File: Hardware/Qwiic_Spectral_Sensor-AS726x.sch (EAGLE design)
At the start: 29 parts, among them J1 Qwiic Right Angle, J2 Serial Interface, J4 Qwiic Right Angle, J5 Flash Programming, U1 IR, U3 4MB Flash

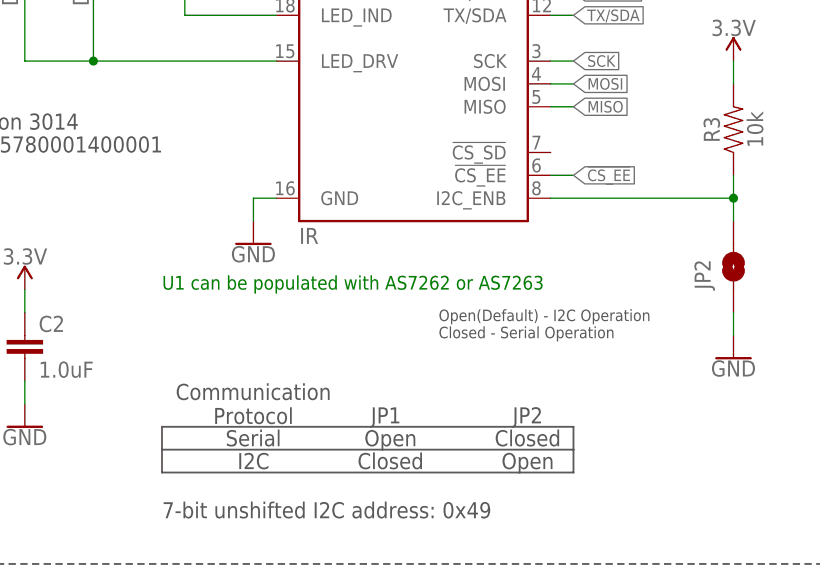
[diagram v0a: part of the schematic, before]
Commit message: Fixed minor borad layout issues
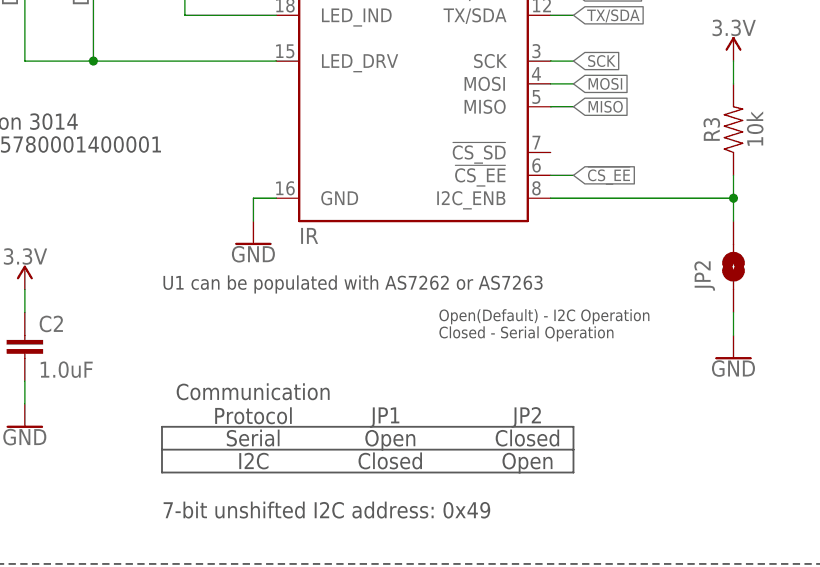
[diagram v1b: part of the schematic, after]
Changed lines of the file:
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@@
 Reset</text>
 <text x="148.59" y="7.112" size="2.54" layer="95">Revised by: Andy England</text>
-<text x="48.26" y="106.68" size="1.524" layer="91">U1 can be populated with AS7262 or AS7263</text>
+<text x="48.26" y="106.68" size="1.524" layer="97">U1 can be populated with AS7262 or AS7263</text>
 </plain>
 <instances>
